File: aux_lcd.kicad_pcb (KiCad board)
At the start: 2 copper layers, 26 x 31 mm, 38 parts, among them P1 DEBUG, P2 LCD, U1 ADXL362, U2 NRF51822, X1 32.768kHz, X2 16Mhz

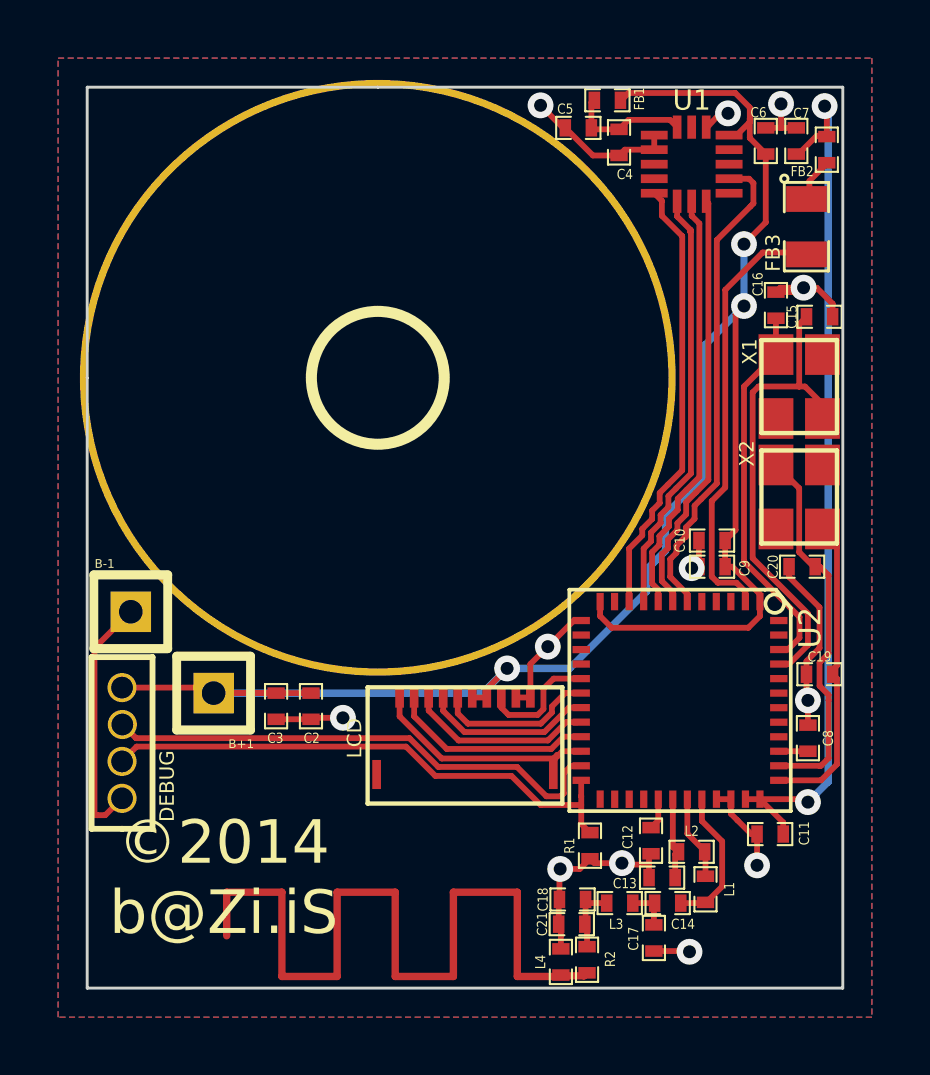
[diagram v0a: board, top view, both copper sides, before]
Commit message: 0.0.2
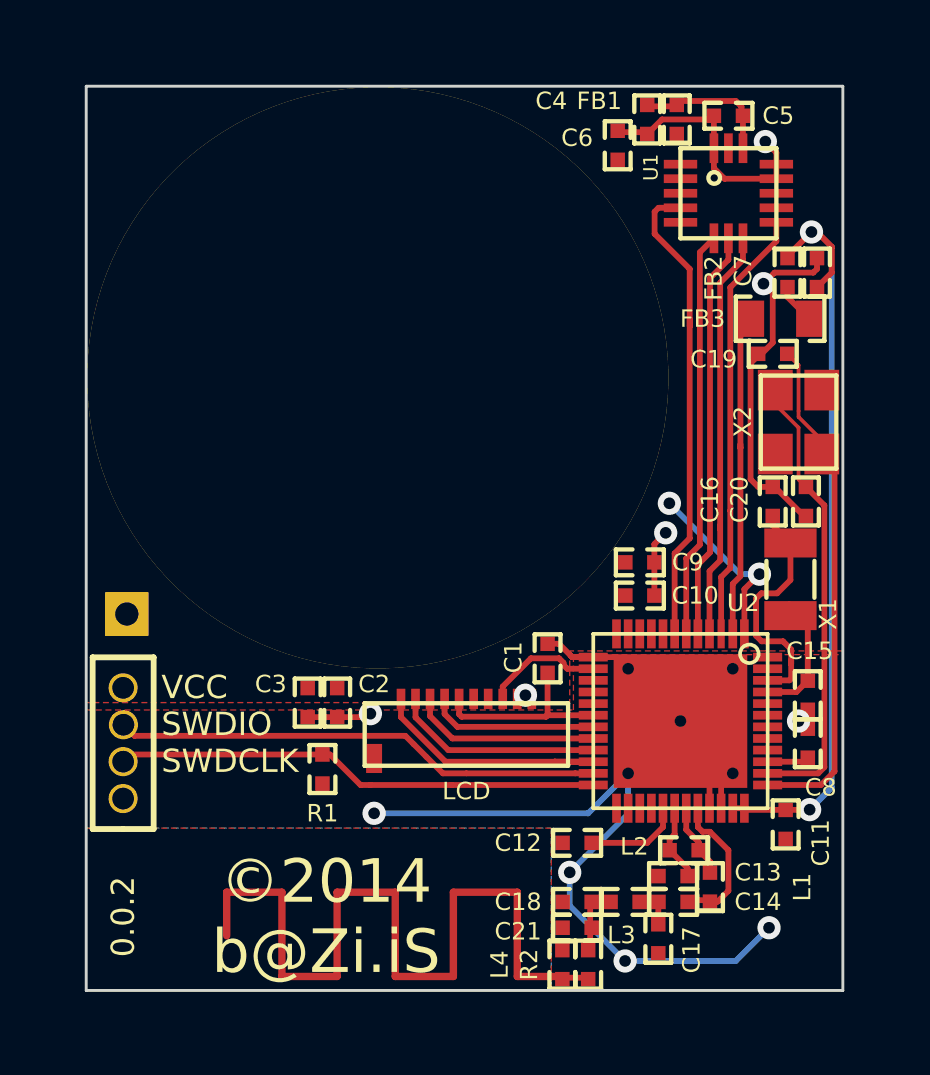
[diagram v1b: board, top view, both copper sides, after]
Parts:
- removed B+1: CONN_1, SIL-1
- added C1: 100nF, Local:SMD-0402_c, F.Cu at (115.8, 119.7)
- B-1: footprint SIL-1 -> Connect:SIL-1
- B1: footprint 1pin -> Local:CR2032
- C10, C11, C12, C13, C14, C15, C16, C17, C18, C19, C2, C20, C21, C3, C4, C5, C6, C7, C8, C9: footprint SM0402_c -> Local:SMD-0402_c
- FB1, FB2, L1, L2, L3, L4: footprint SM0402 -> Local:SMD-0402
- FB3: footprint SM0805 -> Local:smd_0805_r
- P1: footprint 4-PIN-1.27mm -> Local:4-PIN-1.27mm
- R1, R2: footprint SM0402_r -> Local:SMD-0402_r
- U1: footprint LGA16 -> Local:LGA16
- U2: footprint QFN48 -> Local:QFN48
- X1: footprint crystal_FA238-TSX3225 -> Local:FC-13
- X2: footprint crystal_FA238-TSX3225 -> Crystals_Oscillators_SMD:crystal_FA238-TSX3225
- moved C15 13.0 mm to (124.8, 120.9), turned to 270 degrees
- moved C19 11.1 mm to (123.6, 109.2)
- moved R1 9.58 mm to (108.1, 123.5)
- moved C16 6.76 mm to (123.6, 114.3)
- moved X1 6.64 mm to (124.2, 116.9), turned to 90 degrees
- moved C5 5.18 mm to (122.1, 101.0)
- moved C6 5.10 mm to (118.3, 102.0)
- moved C7 4.59 mm to (125.1, 106.4)
- moved FB2 4.44 mm to (124.1, 106.4)
- moved FB3 3.30 mm to (123.8, 108.0), turned to 180 degrees
- moved C10 3.12 mm to (119.0, 117.5), turned to 0 degrees
- moved X2 2.58 mm to (124.5, 111.5)
- moved C12 2.54 mm to (116.9, 126.0), turned to 180 degrees
- moved C9 2.49 mm to (119.0, 116.3), turned to 0 degrees
- moved FB1 2.48 mm to (120.3, 101.1), turned to 90 degrees
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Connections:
- B1 pad 1: GND -> /nRF51822/VCC
- P2 pad 8: /nRF51822/P11 -> /nRF51822/P8
- U1 pad 4: /nRF51822/P2 -> /nRF51822/P3
- U1 pad 6: /nRF51822/P3 -> /nRF51822/P2
- U1 pad 7: /nRF51822/P4 -> /nRF51822/P1
- U1 pad 8: /nRF51822/P5 -> /nRF51822/P0
- U1 pad 9: /nRF51822/P6 -> /nRF51822/P30
- U2 pad 10: /nRF51822/P6 -> (no net)
- U2 pad 14: (no net) -> /nRF51822/P8
- U2 pad 17: /nRF51822/P11 -> (no net)
- U2 pad 3: (no net) -> /nRF51822/P30
- U2 pad 4: (no net) -> /nRF51822/P0
- U2 pad 5: (no net) -> /nRF51822/P1
- U2 pad 8: /nRF51822/P4 -> (no net)
- U2 pad 9: /nRF51822/P5 -> (no net)
- X1 pad 1: /nRF51822/XL2 -> /nRF51822/XL1
- X1 pad 2: /nRF51822/XL1 -> /nRF51822/XL2
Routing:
- net /nRF51822/VCC: track 69.0 -> 7.52 mm, vias 3 -> 2
- net GND: track 46.1 -> 66.1 mm, vias 12 -> 10
- net /nRF51822/P6: track 15.2 -> 0.00 mm
- net /nRF51822/P30: track 0.00 -> 14.9 mm
- net /nRF51822/P5: track 14.7 -> 0.00 mm
- net /nRF51822/P4: track 14.6 -> 0.00 mm
- net /nRF51822/P0: track 0.00 -> 14.2 mm
- net /nRF51822/P1: track 0.00 -> 14.0 mm
- net /nRF51822/XL1: track 16.6 -> 5.07 mm
- net /nRF51822/XC1: track 10.8 -> 17.6 mm
- net /nRF51822/XC2: track 13.1 -> 18.4 mm
- net /nRF51822/P8: track 0.00 -> 4.14 mm
- net /nRF51822/P11: track 4.03 -> 0.00 mm
- net Net-(FB3-Pad2): track 15.1 -> 11.1 mm
- net /nRF51822/XL2: track 13.1 -> 9.24 mm
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- added copper zone on F.Cu, net /nRF51822/VCC
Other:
- board size 26 x 31 mm -> 26 x 31.1 mm
- net class Default: clearance 0.09 -> 0.149; via_dia 0.889 -> 0.8; via_drill 0.635 -> 0.4
- net class Thin added: clearance 0.13, trace_width 0.13, via_dia 0.8, via_drill 0.4
- rule trace_clearance: 0.09 -> 0.149
- rule trace_min: 0.2 -> 0.127
- rule via_min_drill: 0.508 -> 0.4
- rule via_min_size: 0.889 -> 0.8
- board text added: "0.0.2"
- board text added: "SWDCLK"
- board text added: "SWDIO"
- board text added: "VCC"
